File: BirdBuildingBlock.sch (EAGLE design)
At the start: 45 parts, among them CN2 JSTPH, CN3 AMP FCI 10103594-0001LF, U1 UG-2828GDEDF11, U2 MIC5225-3.3v, U3 FAN5331SX, U4 CH340G, U6 MCP73831T-2ACI/OT, Y2 12MHz

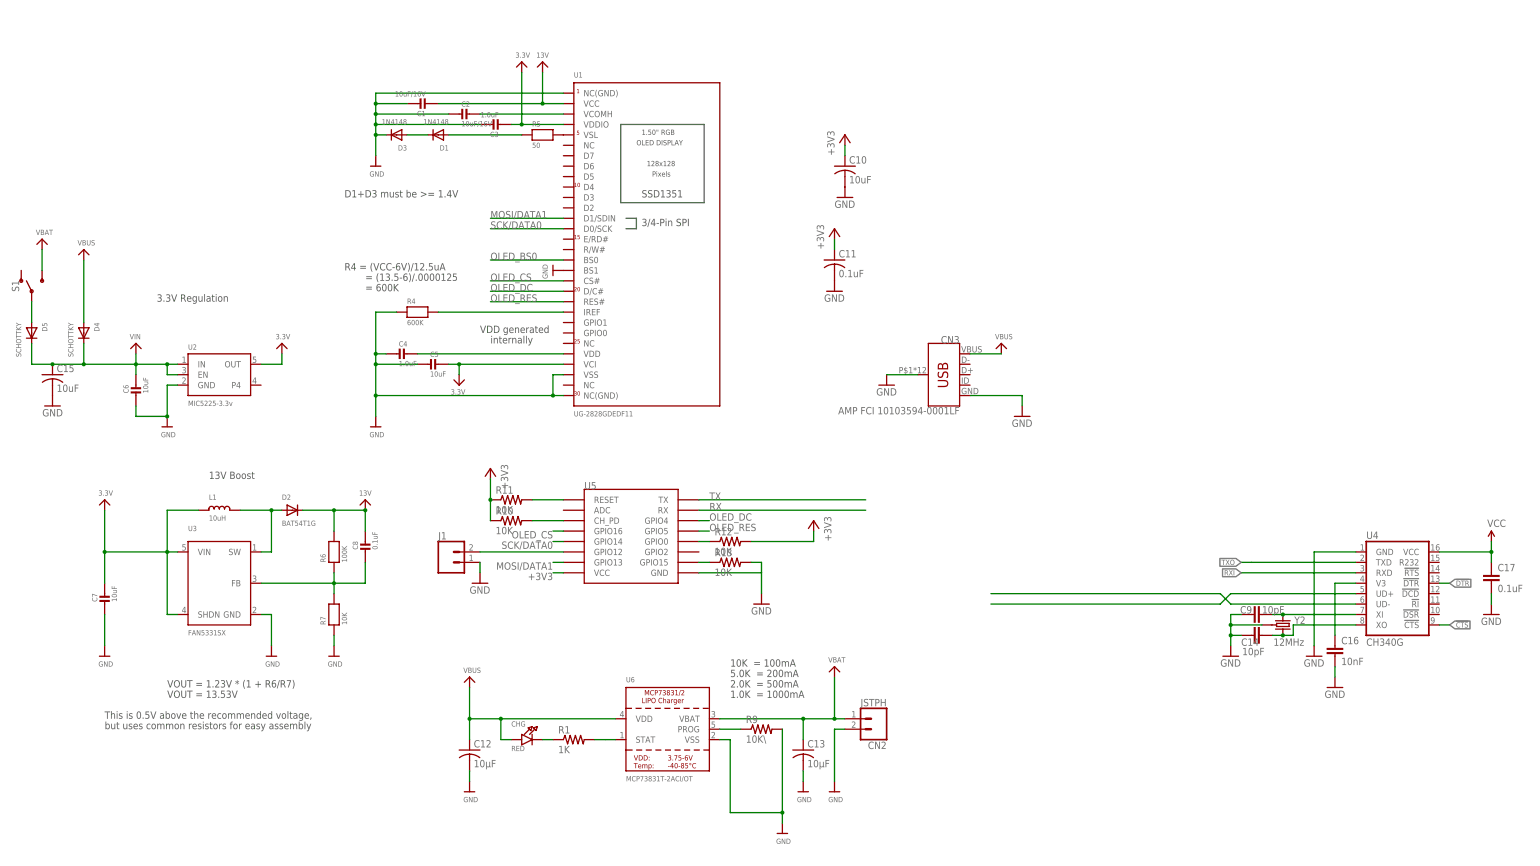
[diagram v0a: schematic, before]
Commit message: Finalizing some circuit design and cleaning up the pcb layout
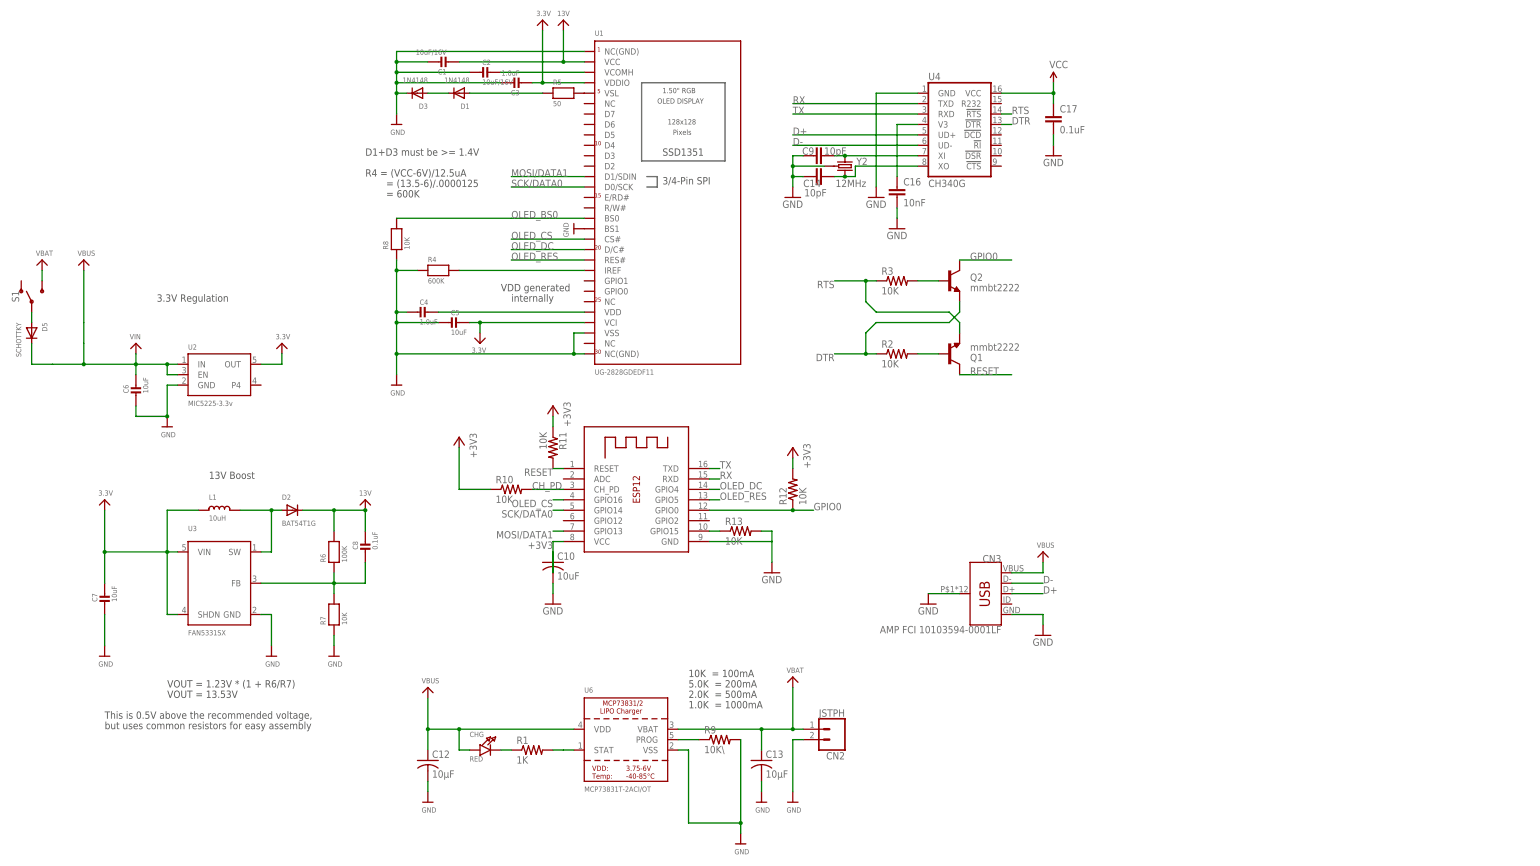
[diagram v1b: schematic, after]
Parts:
- removed C11: 0.1uF, adafruit:C-USC0805
- removed C15: 10uF, adafruit:C-USC0805
- removed D4: SCHOTTKY, adafruit:DIODE_SOD-123FL
- removed J1: (no value), SparkFun-Connectors:CONN_02
- removed U5: (no value), esp8266modules:ESP12SMD
- added Q1, Q2: mmbt2222, SparkFun:TRANSISTOR_NPNSOT23-3
- added R2, R3: 10K, adafruit:R-US_R0603
- added R8: 10K, microbuilder:RESISTOR0805
- added X1: (no value), adafruit:ESP-12
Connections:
- removed net !CTS: U4.!CTS
- removed net !DTR: U4.!DTR
- removed net N$15: R12.1, U5.GPIO0
- removed net N$16: R10.2, U5.CH_PD
- removed net N$18: J1.2, U5.GPIO12
- removed net N$2: R11.2, U5.RESET
- removed net RXI: U4.RXD
- removed net TXO: U4.TXD
- removed net VIN: C15.1, C6.P$1, D4.C, D5.C, U2.EN, U2.IN
- new net CH_PD: R10.2, X1.CH_PD
- new net D+: CN3.D+, U4.UD+
- new net D-: CN3.D-, U4.UD-
- new net DTR: Q2.E, R2.1, U4.!DTR
- new net GPIO0: Q2.C, R12.1, X1.GPIO0
- new net RESET: Q1.C, R11.2, X1.RESET
- new net RTS: Q1.E, R3.1, U4.!RTS
- net +3V3: now also X1.VCC; no longer C11.1, U5.VCC
- net GND: now also R8.1, X1.GND; no longer C11.2, C15.2, J1.1, U5.GND
- net MOSI/DATA1: now also X1.GPIO13; no longer U5.GPIO13
- net N$13: now also Q1.B, R2.2; no longer U4.UD-
- net N$14: now also Q2.B, R3.2; no longer U4.UD+
- net N$17: now also X1.GPIO15; no longer U5.GPIO15
- net OLED_BS0: now also R8.2
- net OLED_CS: now also X1.GPIO16; no longer U5.GPIO16
- net OLED_DC: now also X1.GPIO4; no longer U5.GPIO4
- net OLED_RES: now also X1.GPIO5; no longer U5.GPIO5
- net RX: now also U4.TXD, X1.RXD; no longer U5.RX
- net SCK/DATA0: now also X1.GPIO14; no longer U5.GPIO14
- net TX: now also U4.RXD, X1.TXD; no longer U5.TX
- net VBUS: now also C6.P$1, D5.C, U2.EN, U2.IN; no longer D4.A
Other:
- moved on the sheet: C1, C10, C12, C13, C14, C16, C17, C2, C3, C4, C5, C9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
